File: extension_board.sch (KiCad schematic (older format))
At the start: 37 parts, among them CN1 Conn_02x20_Odd_Even, CN11 Conn_02x05_Odd_Even, CN12 Conn_02x20_Odd_Even, J1 Screw_Terminal_01x02, J2 Conn_01x02, J3 Conn_01x02, J4 Conn_01x02, J5 Conn_02x03_Odd_Even, J6 Conn_01x02, J7 Conn_02x14_Odd_Even, U1 LM334Z, U2 LM334Z, U3 LM334Z, U4 LM334Z

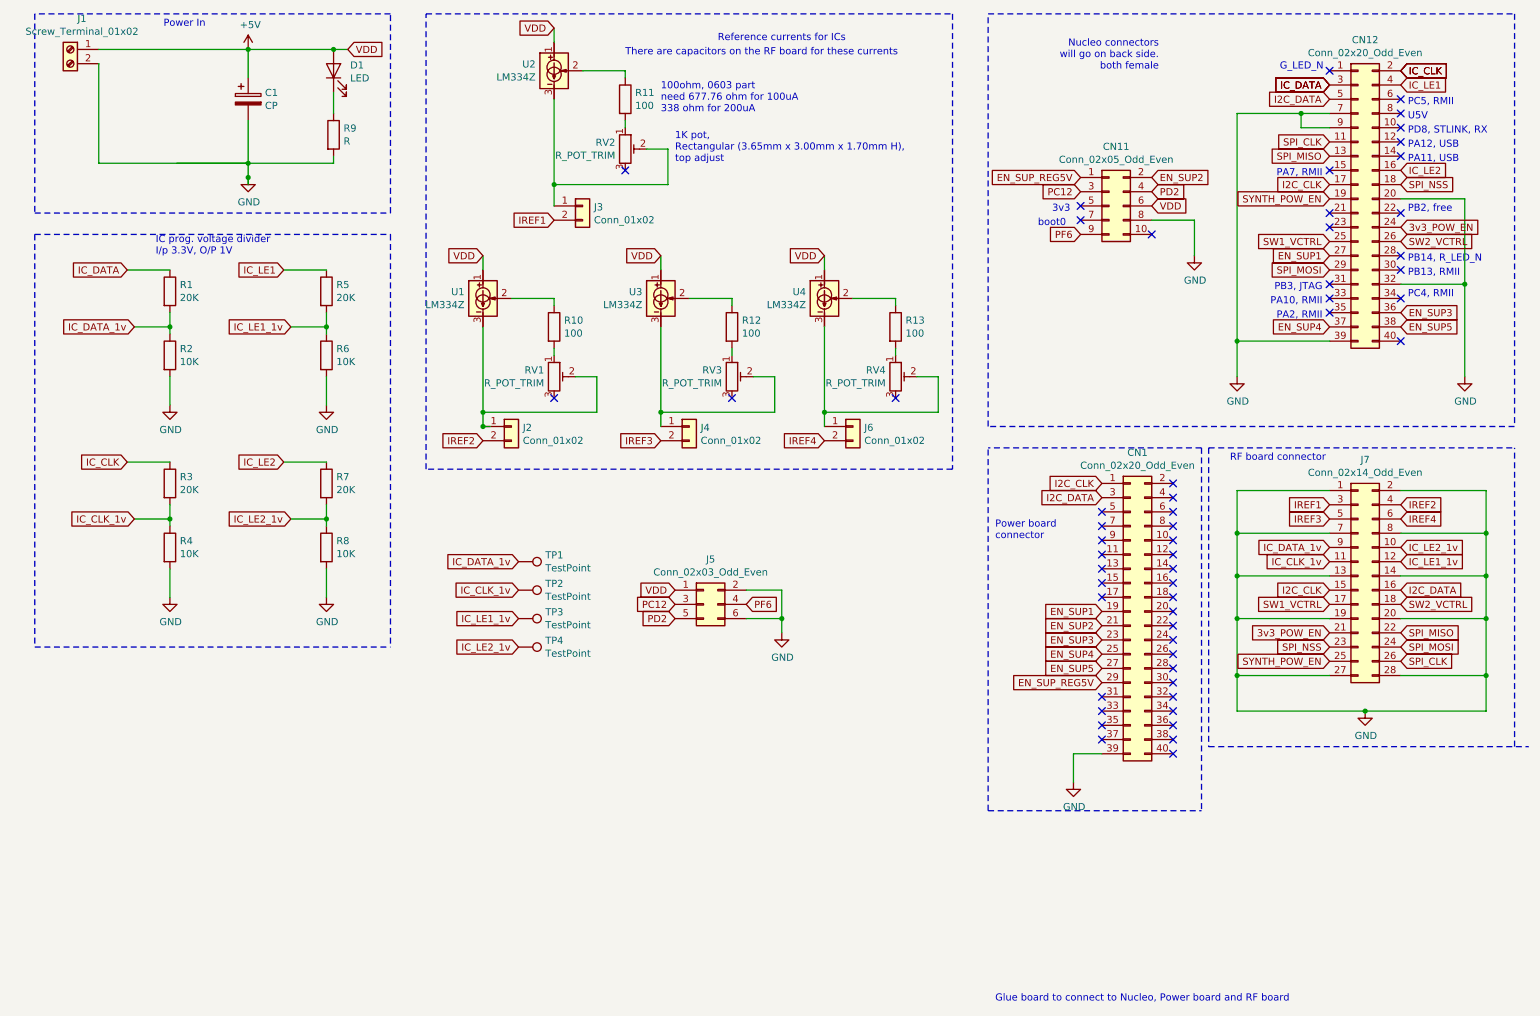
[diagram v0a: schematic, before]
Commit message: first version of the pcb
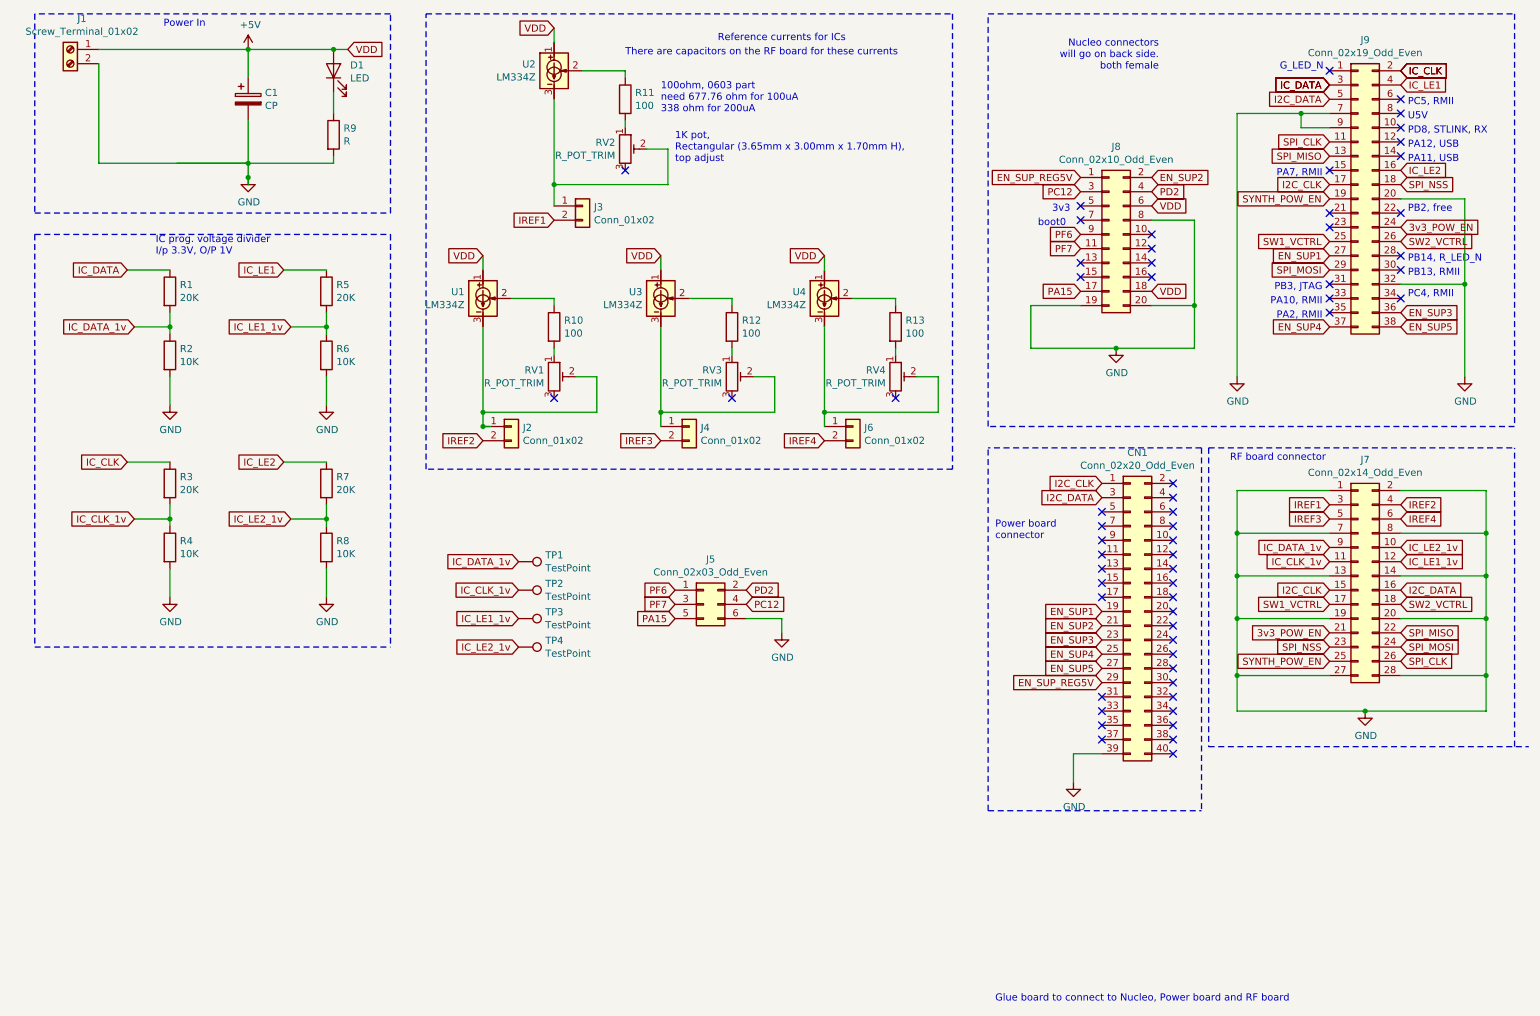
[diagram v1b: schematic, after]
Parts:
- removed CN11: Conn_02x05_Odd_Even, symbol Connector_Generic:Conn_02x05_Odd_Even
- removed CN12: Conn_02x20_Odd_Even, symbol Connector_Generic:Conn_02x20_Odd_Even
- added J8: Conn_02x10_Odd_Even, Connector_PinHeader_2.54mm:PinHeader_2x10_P2.54mm_Vertical, symbol Connector_Generic:Conn_02x10_Odd_Even
- added J9: Conn_02x19_Odd_Even, Connector_PinHeader_2.54mm:PinHeader_2x19_P2.54mm_Vertical, symbol Connector_Generic:Conn_02x19_Odd_Even
- C1: footprint (none) -> Capacitor_SMD:CP_Elec_4x5.8
- CN1: footprint (none) -> Connector_PinHeader_2.54mm:PinHeader_2x20_P2.54mm_Vertical_SMD
- D1: footprint (none) -> LED_SMD:LED_0805_2012Metric_Pad1.15x1.40mm_HandSolder
- J1: footprint (none) -> digikey-footprints:Term_Block_1x2_P5.08MM
- J2, J3, J4, J6: footprint (none) -> Connector_PinHeader_2.54mm:PinHeader_2x01_P2.54mm_Vertical_SMD
- J5: footprint (none) -> Connector_PinHeader_2.54mm:PinHeader_2x03_P2.54mm_Vertical_SMD
- J7: footprint (none) -> Connector_PinHeader_2.54mm:PinHeader_2x14_P2.54mm_Vertical_SMD
- R1, R2, R3, R4, R5, R6, R7, R8, R9: footprint (none) -> Resistor_SMD:R_0805_2012Metric_Pad1.15x1.40mm_HandSolder
- RV1, RV2, RV3, RV4: footprint (none) -> digikey-footprints:Trimpot_3.8mmx3.6mm_TC33X-2-103E
- TP1, TP2, TP3, TP4: footprint (none) -> TestPoint:TestPoint_Pad_2.5x2.5mm
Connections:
- net labels added: PA15, PF7
- wire segments 111 -> 113
- no-connect marks 55 -> 59
